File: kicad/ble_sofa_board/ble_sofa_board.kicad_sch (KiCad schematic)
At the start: 17 parts, among them J1 Screw_Terminal_01x02, J2 Screw_Terminal_01x02, J3 Screw_Terminal_01x02, J4 Screw_Terminal_01x02, J5 Screw_Terminal_01x02, J6 Screw_Terminal_01x02, J7 RJ9, U1 LM2596S_Buck_Module, U2 LM2596S_Buck_Module, U3 Pico_Dual_Channel_Relay_HAT

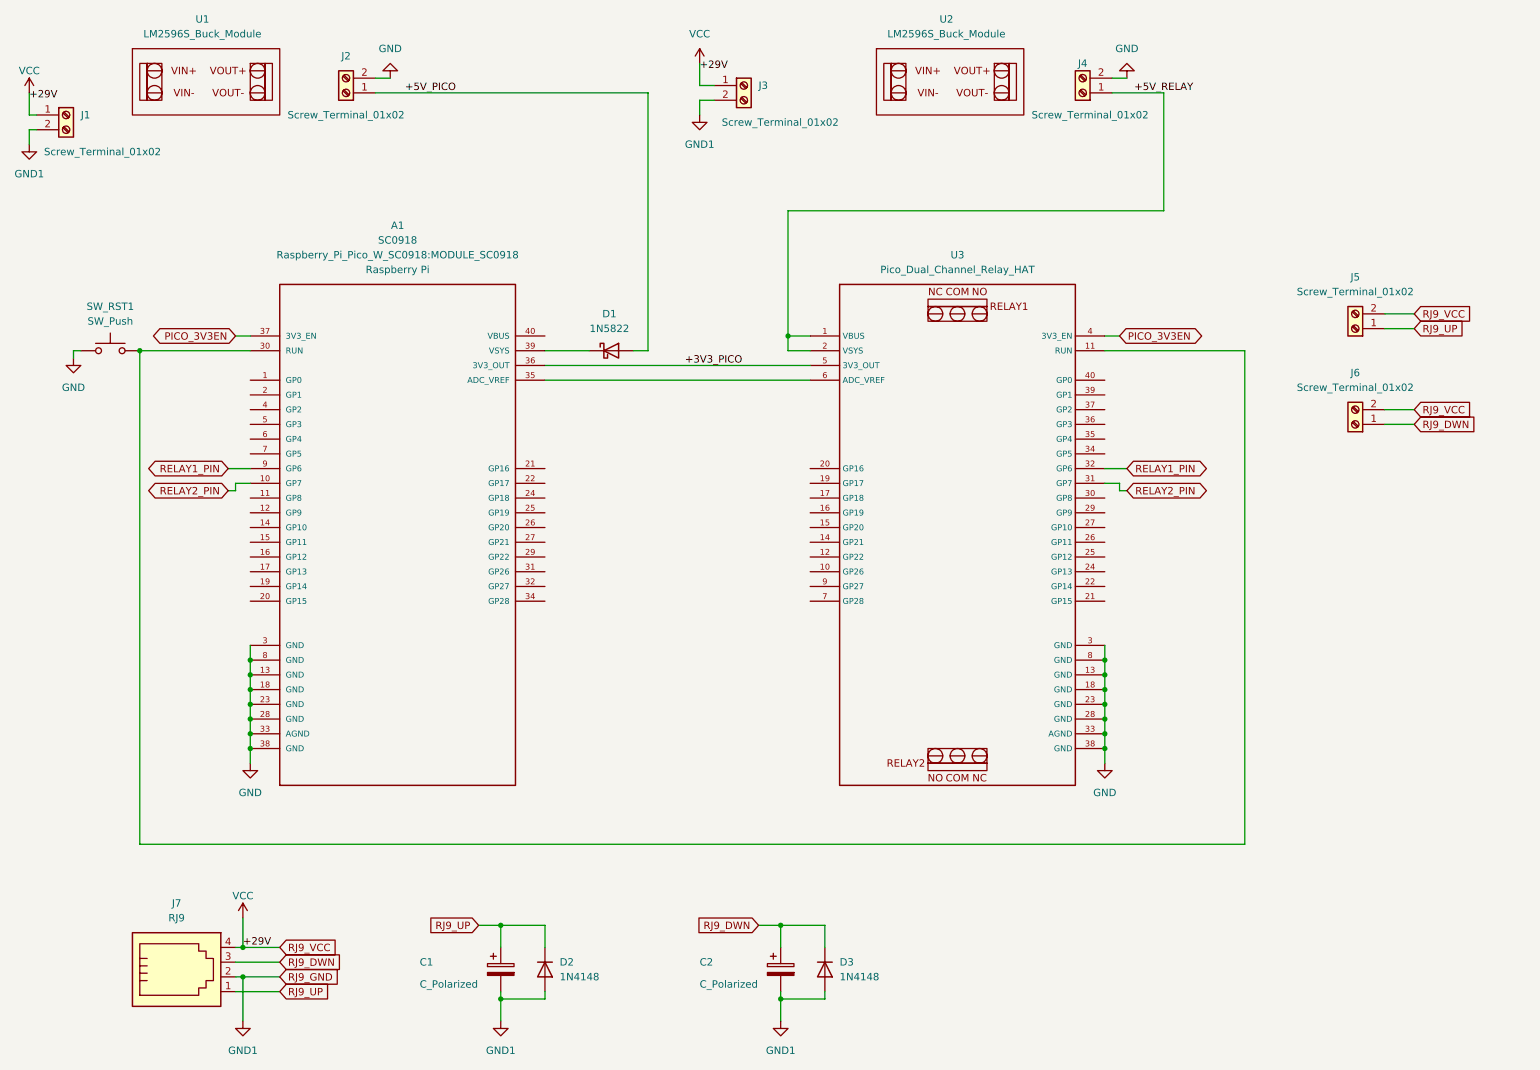
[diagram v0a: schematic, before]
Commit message: ble_sofa_app - Update schematic
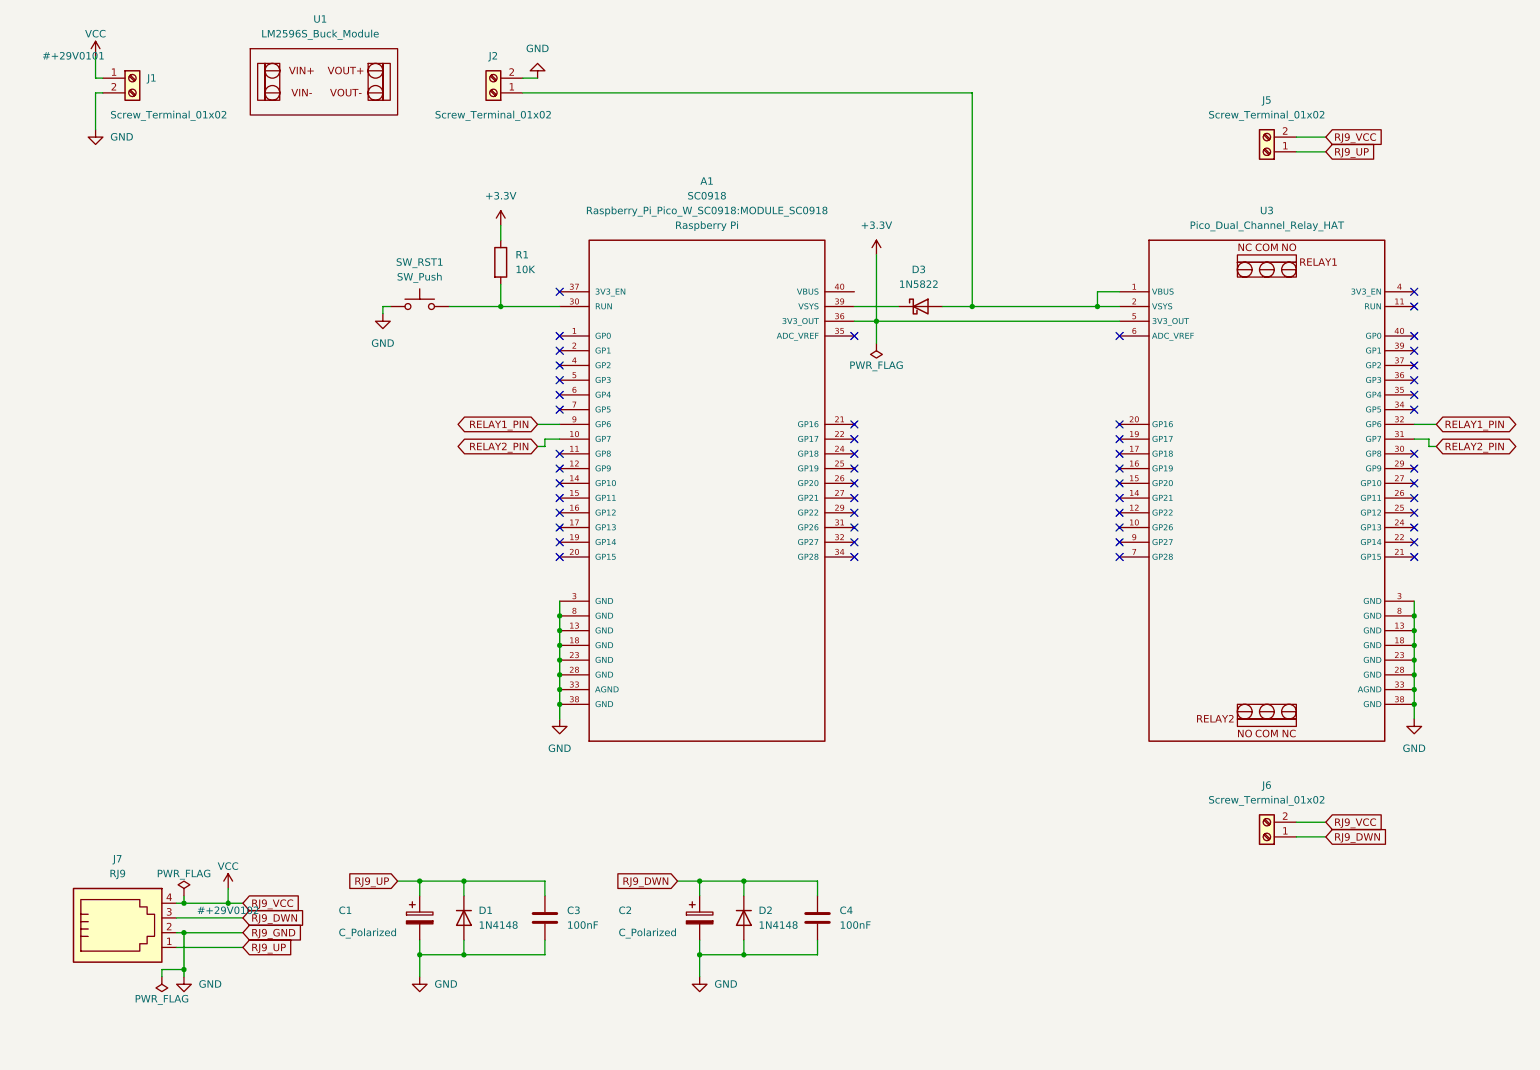
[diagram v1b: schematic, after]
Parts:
- removed J3, J4: Screw_Terminal_01x02, TerminalBlock:TerminalBlock_bornier-2_P5.08mm, symbol Connector:Screw_Terminal_01x02
- removed U2: LM2596S_Buck_Module, AZ_Delivery:LM2596S_Buck_Module, symbol AZ_Delivery:LM2596S_Buck_Module
- added C3, C4: 100nF, symbol Device:C
- added R1: 10K, symbol Device:R
- renumbered D2 to D1, D3 to D2, D1 to D3
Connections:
- net +5V_RELAY is gone; now on an unnamed net: U3.1 (VBUS), U3.2 (VSYS)
- net GND1 is gone; now on net GND: C1.2, C2.2, D1.2 (A), D2.2 (A), J1.2 (Pin_2), J7.2
- net GND: now also C3.2, C4.2
- net RJ9_DWN: now also C4.1
- net RJ9_UP: now also C3.1
- net at A1.30 (RUN), SW_RST1.2: now also R1.2; no longer U3.11 (RUN)
- net at A1.35 (ADC_VREF): no longer U3.6 (ADC_VREF)
- net +3V3_PICO renamed +3V3
- net +3V3: now also R1.1
- net +5V_PICO: no longer names the net of D3.2 (A), J2.1 (Pin_1)
- net PICO_3V3EN: no longer names the net of A1.37 (3V3_EN)
- net PICO_3V3EN: no longer U3.4 (3V3_EN)
- no-connect marks 0 -> 53
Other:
- moved on the sheet: A1, C1, C2, D1, D2, D3, J1, J2, J5, J6, J7, SW_RST1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
